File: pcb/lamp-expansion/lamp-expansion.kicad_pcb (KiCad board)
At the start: 2 copper layers, 139.7 x 46.2 mm, 77 parts, among them IC1 PAM2421, IC2 MCP73811, IC3 NTHD3101F, IC6 LM1117_5.0, IC7 FT230X_SOP, IC9 CC3000, J1 MICROUSB, J2 DCIN, J3 SERIAL, J4 5PIN_INPUT, J5 2PIN_POWER, J7 2PIN_POWER, J8 AVR_ISP, J9 UF.L, Q1 2N7002

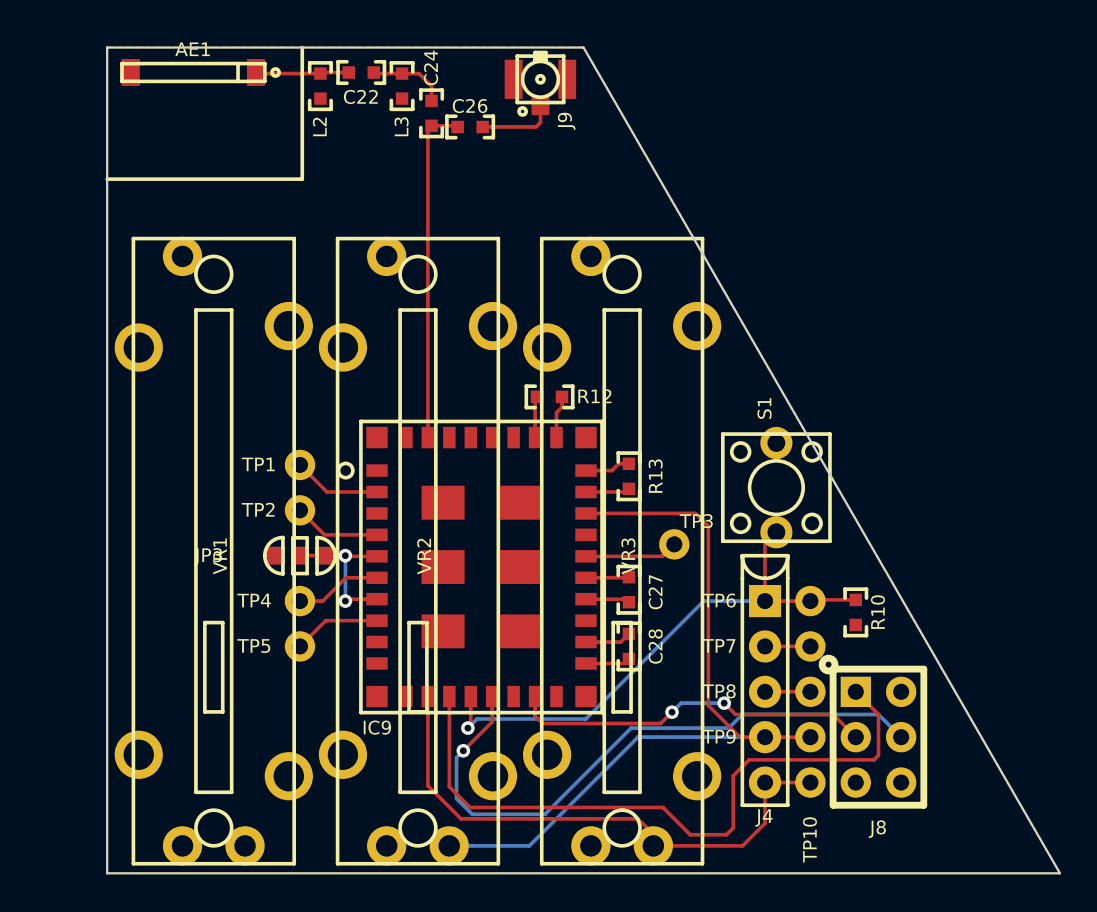
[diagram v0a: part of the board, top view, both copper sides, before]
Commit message: last few traces
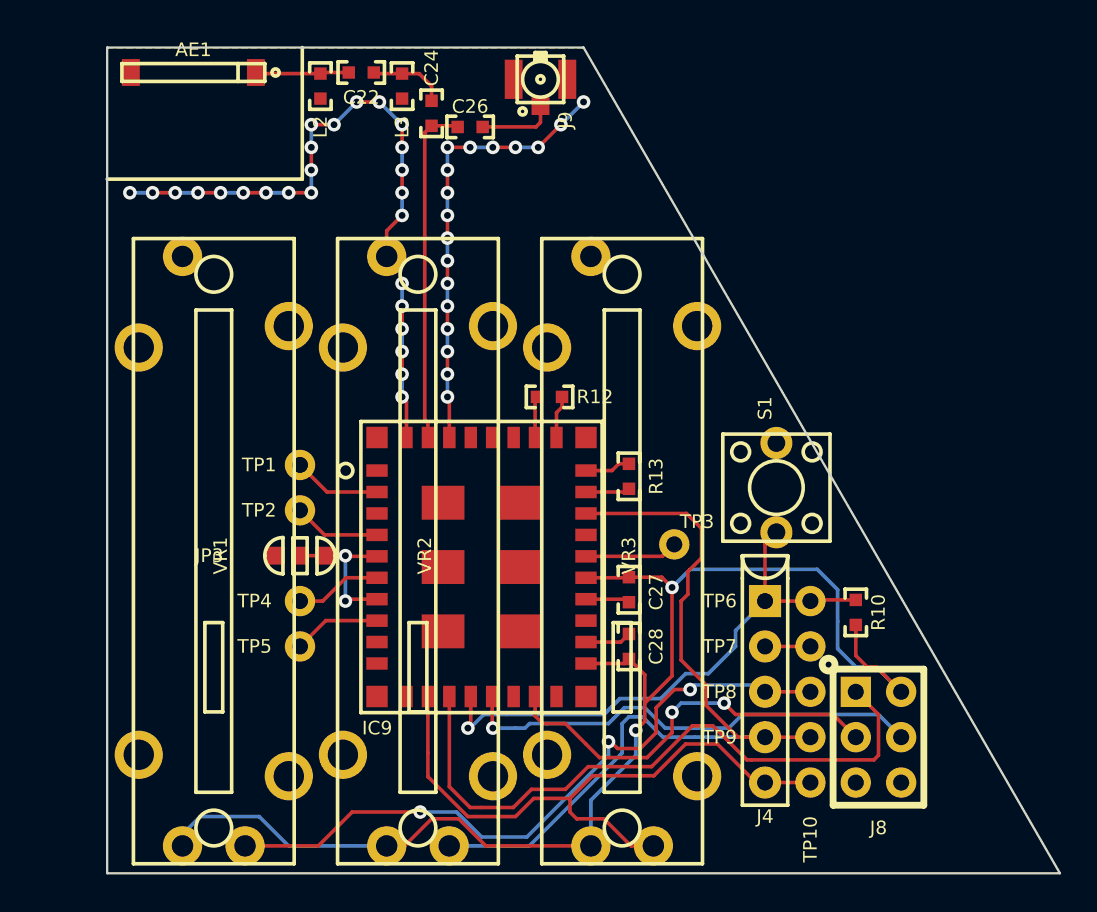
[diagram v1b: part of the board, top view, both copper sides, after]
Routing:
- net VCC: track 4.93 -> 76.3 mm, vias 0 -> 2
- net GND: track 100.3 -> 161.8 mm, vias 17 -> 61
- net /POT_0: track 2.54 -> 38.3 mm, vias 0 -> 3
- net /CC_MOSI: track 34.6 -> 26.4 mm
- net /CC_SEL: track 31.0 -> 35.6 mm
- net /CC_EN: track 43.8 -> 46.5 mm
- net /CC_SCK: track 20.5 -> 22.7 mm
- net /CC_MISO: track 37.8 -> 36.4 mm
- net /CC_IRQ: track 30.6 -> 31.2 mm
